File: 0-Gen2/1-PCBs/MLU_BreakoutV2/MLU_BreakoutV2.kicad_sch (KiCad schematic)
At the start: 17 parts, among them J13 SBH11-PBPC-D10-ST-BK, J7 SBH11-PBPC-D10-ST-BK, U6 Teensy4.1

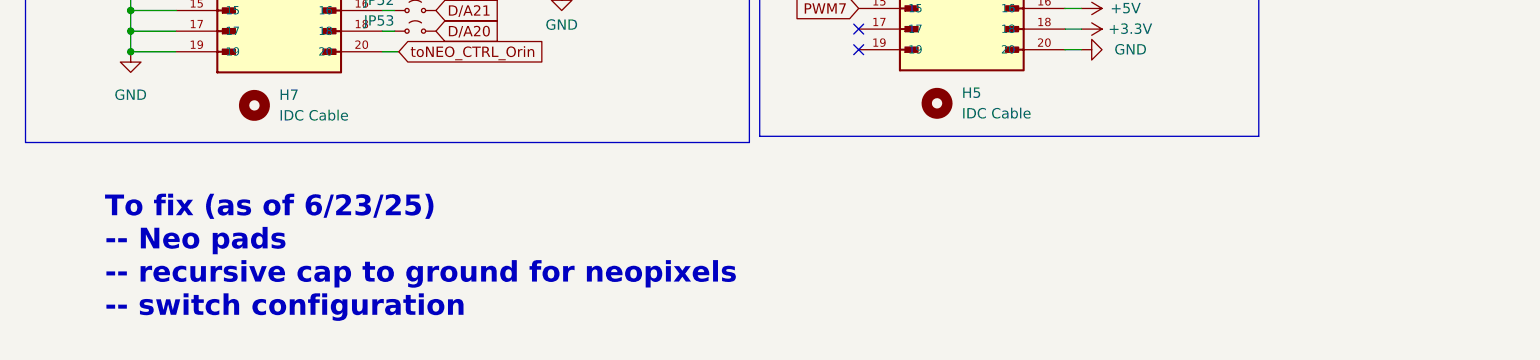
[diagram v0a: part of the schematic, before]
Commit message: pushing after comp
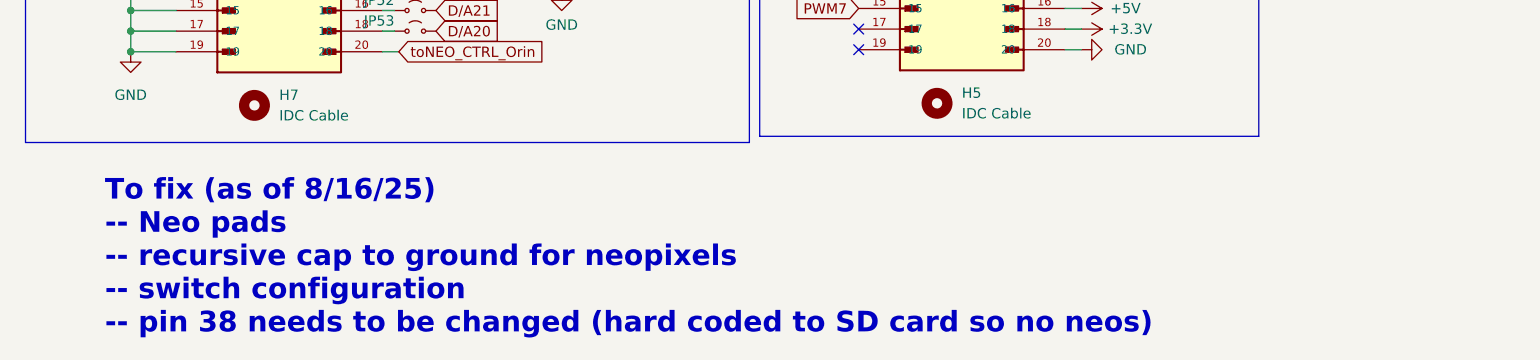
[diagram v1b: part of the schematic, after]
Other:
- note added: "To fix (as of 8/16/25) -- Neo pads -- recursive cap to ground for neopixels -- switch configuration -- pin 38 needs to be changed (hard coded to SD card so no neos)"
- note removed: "To fix (as of 6/23/25) -- Neo pads -- recursive cap to ground for neopixels -- switch configuration"
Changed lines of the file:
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@@
 		)
 	)
-	(text "To fix (as of 6/23/25)\n-- Neo pads\n-- recursive cap to ground for neopixels\n-- switch configuration"
+	(text "To fix (as of 8/16/25)\n-- Neo pads\n-- recursive cap to ground for neopixels\n-- switch configuration\n-- pin 38 needs to be changed (hard coded to SD card so no neos)"
 		(exclude_from_sim no)
 		(at 24.765 176.2125 0)
